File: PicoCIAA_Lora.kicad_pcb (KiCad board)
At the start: 2 copper layers, 47 x 30 mm, 11 parts, among them P1 EDGE_SMA, P3 PWR, P4 MOUNTING_HOLE, P5 MOUNTING_HOLE, P6 IO1, P8 IO3, U1 RFM95

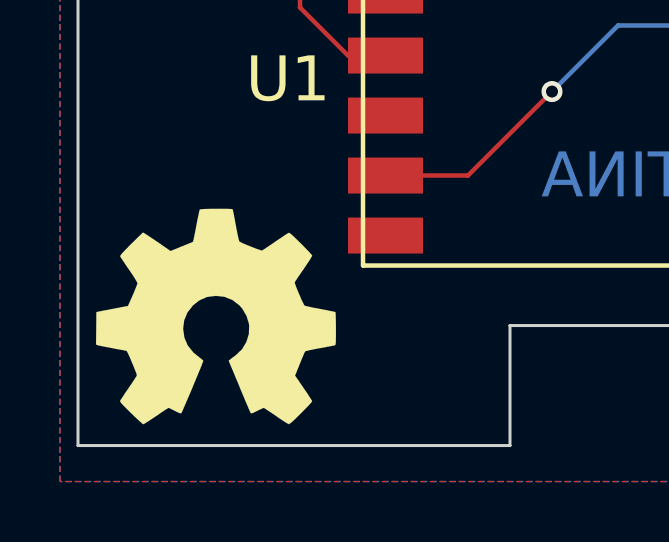
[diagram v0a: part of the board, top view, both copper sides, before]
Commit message: DRC: Prueba
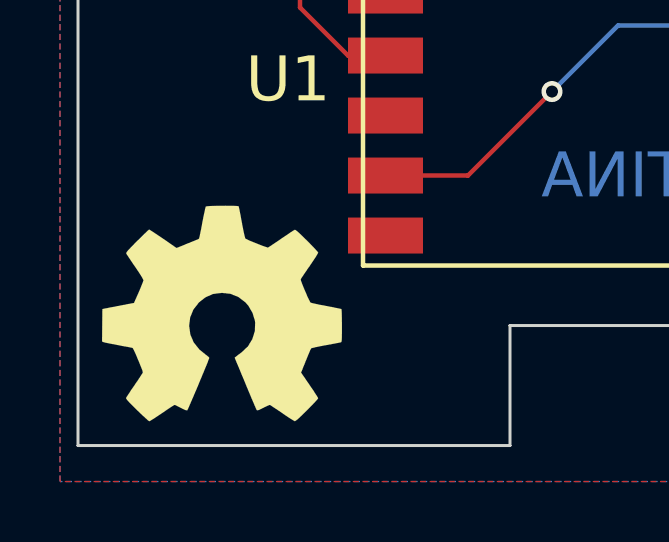
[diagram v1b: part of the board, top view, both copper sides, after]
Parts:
- G101: footprint ej2cese:Logo_OSHWA -> footprints:Logo_OSHWA
- moved G101 0.22 mm to (57.8, 125.6)
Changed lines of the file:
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@@
     )
   )
-  (module ej2cese:Logo_OSHWA (layer F.Cu)
-    (at 57.6 125.7)
-    (fp_text reference G101 (at 0 3.3) (layer F.SilkS) hide
+  (module Fiducials:Fiducial_1mm_Dia_2.54mm_Outer_CopperTop (layer F.Cu)
+    (at 55.8 102.7)
+    (descr "Circular Fiducial, 1mm bare copper top; 2.54mm keepout")
+    (tags marker)
+    (attr virtual)
+    (fp_text reference REF1 (at -0.1 2.3) (layer F.SilkS)
+      (effects (font (size 1 1) (thickness 0.15)))
+    )
+    (fp_text value F1 (at 0 -1.8) (layer F.Fab)
+      (effects (font (size 1 1) (thickness 0.15)))
+    )
+    (fp_circle (center 0 0) (end 1.55 0) (layer F.CrtYd) (width 0.05))
+    (pad ~ smd circle (at 0 0) (size 1 1) (layers F.Cu F.Mask)
+      (solder_mask_margin 0.77) (clearance 0.77))
+  )
+  (module Fiducials:Fiducial_1mm_Dia_2.54mm_Outer_CopperTop (layer F.Cu)
+    (at 91.6 124.4)
+    (descr "Circular Fiducial, 1mm bare copper top; 2.54mm keepout")
+    (tags marker)
+    (attr virtual)
+    (fp_text reference REF2 (at 0.5 2.4) (layer F.SilkS)
+      (effects (font (size 1 1) (thickness 0.15)))
+    )
+    (fp_text value F2 (at 0 -1.8) (layer F.Fab)
+      (effects (font (size 1 1) (thickness 0.15)))
+    )
+    (fp_circle (center 0 0) (end 1.55 0) (layer F.CrtYd) (width 0.05))
+    (pad ~ smd circle (at 0 0) (size 1 1) (layers F.Cu F.Mask)
+      (solder_mask_margin 0.77) (clearance 0.77))
+  )
+  (module footprints:Logo_OSHWA (layer F.Cu)
+    (at 57.8 125.6)
+    (fp_text reference G101 (at 0 3.2) (layer F.SilkS) hide
       (effects (font (size 0.7112 0.4572) (thickness 0.1143)))
     )
-    (fp_text value Logo_OSHWA (at -2.6 -3.6) (layer F.SilkS) hide
+    (fp_text value Logo_OSHWA (at -2.6 -3.4) (layer F.SilkS) hide
       (effects (font (size 0.36322 0.36322) (thickness 0.07112)))
     )
@@
       (xy -2.42316 3.59156)) (layer F.SilkS) (width 0.00254))
   )
-  (module Fiducials:Fiducial_1mm_Dia_2.54mm_Outer_CopperTop (layer F.Cu)
-    (at 55.8 102.7)
-    (descr "Circular Fiducial, 1mm bare copper top; 2.54mm keepout")
-    (tags marker)
-    (attr virtual)
-    (fp_text reference REF1 (at -0.1 2.3) (layer F.SilkS)
-      (effects (font (size 1 1) (thickness 0.15)))
-    )
-    (fp_text value F1 (at 0 -1.8) (layer F.Fab)
-      (effects (font (size 1 1) (thickness 0.15)))
-    )
-    (fp_circle (center 0 0) (end 1.55 0) (layer F.CrtYd) (width 0.05))
-    (pad ~ smd circle (at 0 0) (size 1 1) (layers F.Cu F.Mask)
-      (solder_mask_margin 0.77) (clearance 0.77))
-  )
-  (module Fiducials:Fiducial_1mm_Dia_2.54mm_Outer_CopperTop (layer F.Cu)
-    (at 91.6 124.4)
-    (descr "Circular Fiducial, 1mm bare copper top; 2.54mm keepout")
-    (tags marker)
-    (attr virtual)
-    (fp_text reference REF2 (at 0.5 2.4) (layer F.SilkS)
-      (effects (font (size 1 1) (thickness 0.15)))
-    )
-    (fp_text value F2 (at 0 -1.8) (layer F.Fab)
-      (effects (font (size 1 1) (thickness 0.15)))
-    )
-    (fp_circle (center 0 0) (end 1.55 0) (layer F.CrtYd) (width 0.05))
-    (pad ~ smd circle (at 0 0) (size 1 1) (layers F.Cu F.Mask)
-      (solder_mask_margin 0.77) (clearance 0.77))
-  )
   (gr_text "IND. ARGENTINA" (at 77 121) (layer B.Cu)
